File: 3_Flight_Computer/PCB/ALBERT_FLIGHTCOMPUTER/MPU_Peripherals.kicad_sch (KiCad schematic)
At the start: 27 parts, among them IC3 PCA9685PW,118, IC4 W25N01GVZEIG, J10 Screw_Terminal_01x02, J11 Screw_Terminal_01x02, J5 Conn_02x08_Odd_Even, J6 Conn_01x08, J8 Screw_Terminal_01x02, J9 Screw_Terminal_01x02, Q1 BSC028N06LS3, Q2 BSC028N06LS3, Q3 BSC028N06LS3, Q4 BSC028N06LS3

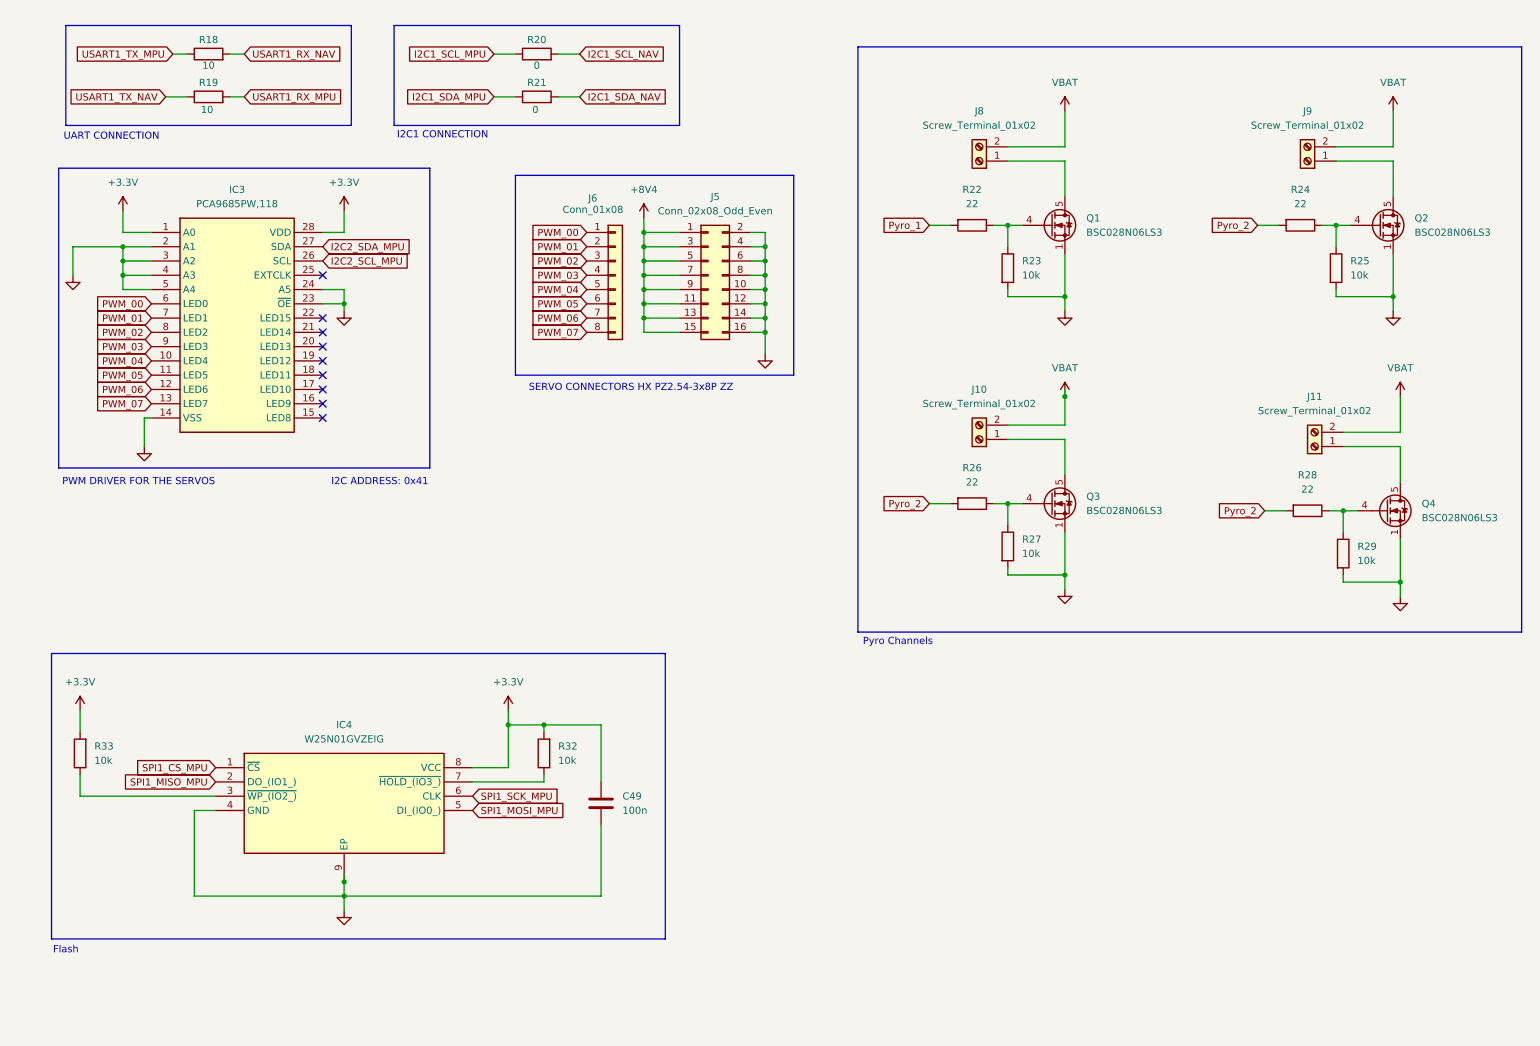
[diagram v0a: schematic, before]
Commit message: Refactor code structure for improved readability and maintainability
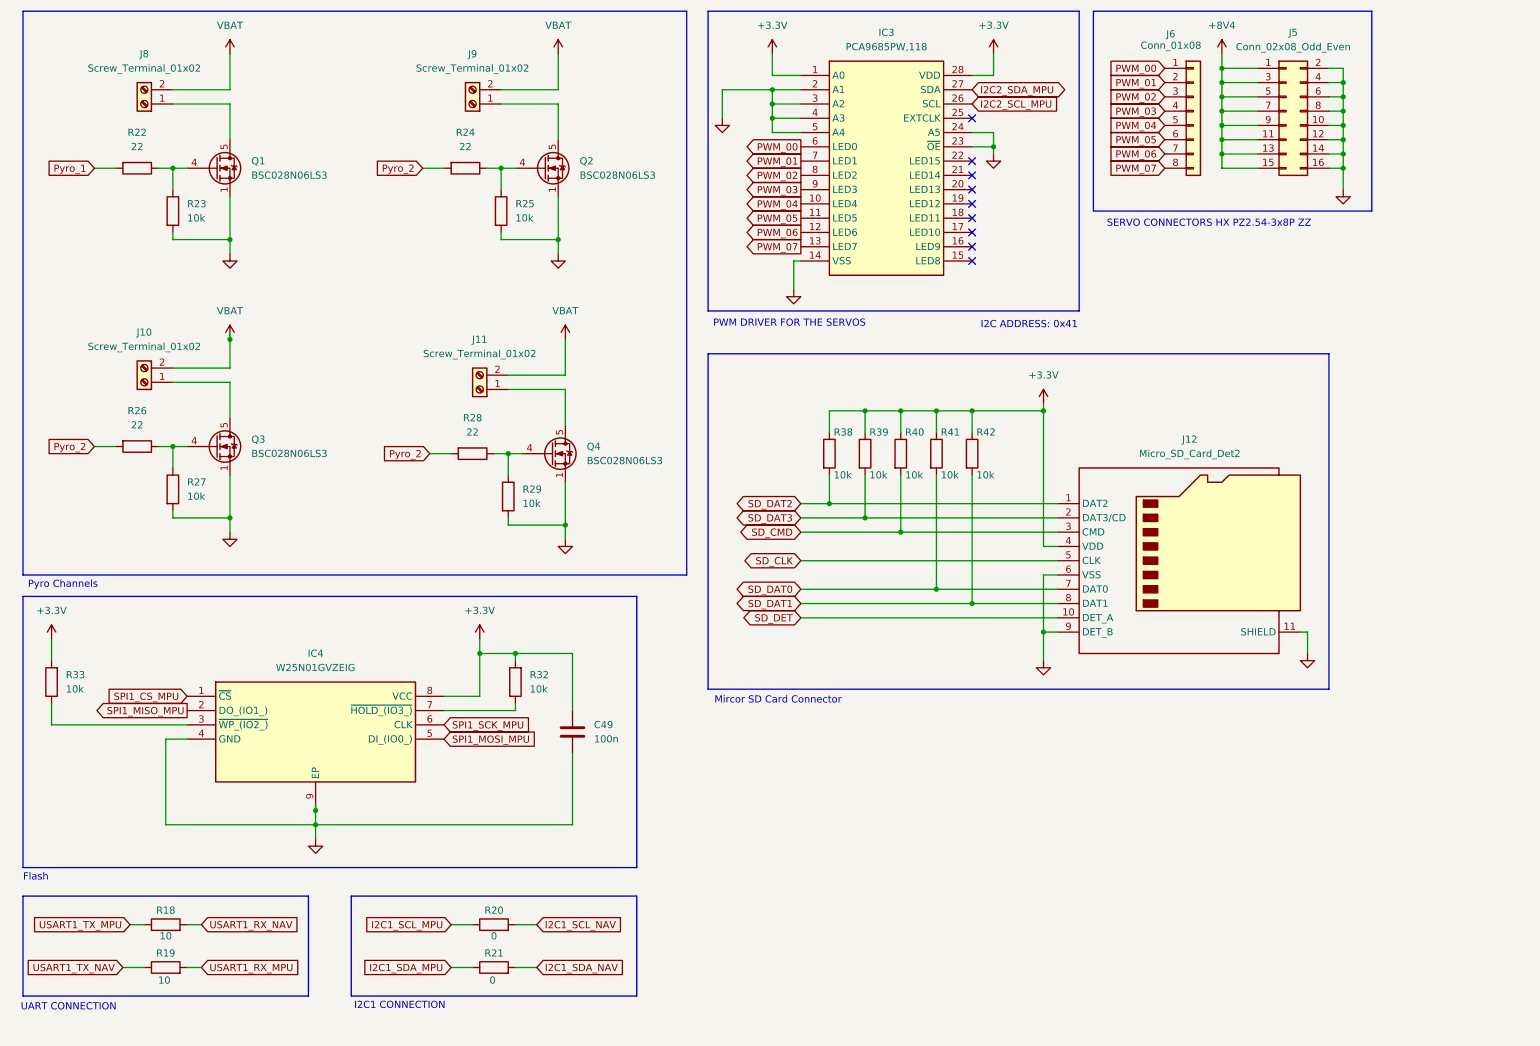
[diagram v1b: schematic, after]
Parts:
- added J12: Micro_SD_Card_Det2, Connector_Card:microSD_HC_Hirose_DM3AT-SF-PEJM5, symbol Connector:Micro_SD_Card_Det2
- added R38, R39, R40, R41, R42: 10k, symbol Device:R
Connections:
- net +3.3V: now also J12.4 (VDD), R38.1, R39.1, R40.1, R41.1, R42.1
- net GND: now also J12.11 (SHIELD), J12.6 (VSS), J12.9 (DET_B)
- new net SD_CLK: J12.5 (CLK)
- new net SD_CMD: J12.3 (CMD), R40.2
- new net SD_DAT0: J12.7 (DAT0), R41.2
- new net SD_DAT1: J12.8 (DAT1), R42.2
- new net SD_DAT2: J12.1 (DAT2), R38.2
- new net SD_DAT3: J12.2 (DAT3/CD), R39.2
- new net SD_DET: J12.10 (DET_A)
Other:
- note added: "Mircor SD Card Connector"
- title: (none) -> MPU Peripherals
- moved on the sheet: C49, IC3, IC4, J10, J11, J5, J6, J8, J9, Q1, Q2, Q3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

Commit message: Add lock file for ALBERT_FLIGHTCOMPUTER PCB design
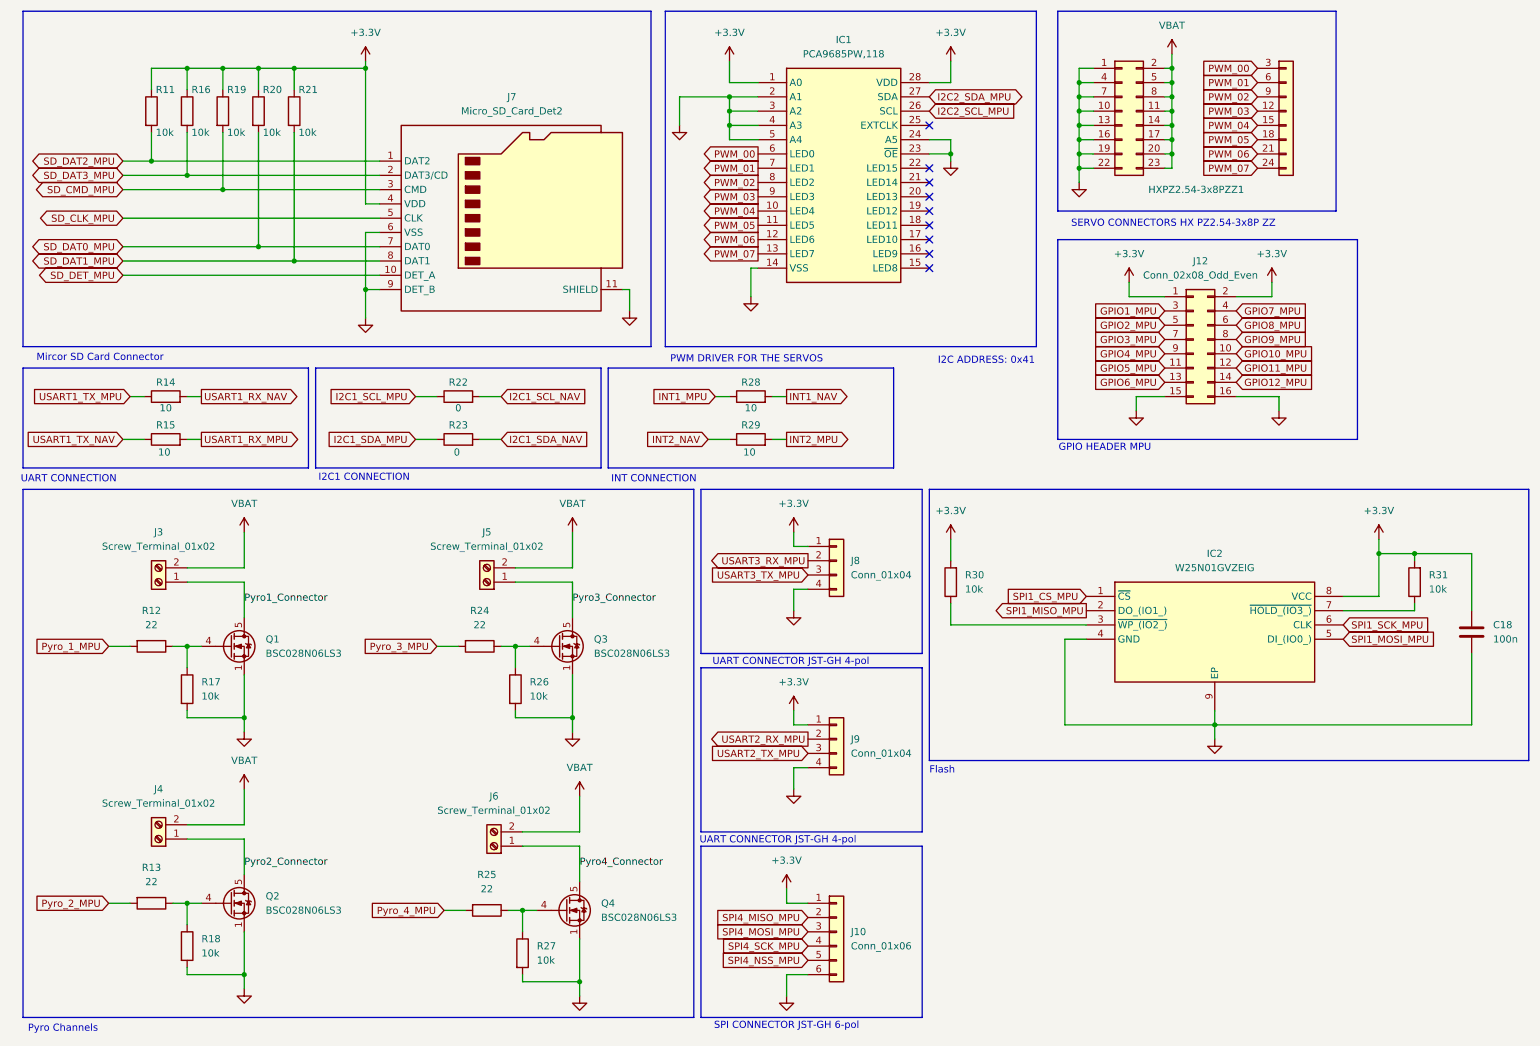
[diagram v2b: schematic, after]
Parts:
- removed J5: Conn_02x08_Odd_Even, symbol Connector_Generic:Conn_02x08_Odd_Even
- removed J6: Conn_01x08, symbol Connector_Generic:Conn_01x08
- added HXPZ2.54-3x8PZZ1: ~, HXPZ2.54-3x8PZZ:HX PZ2.54-3x8P ZZ, symbol HXPZ2.54-3x8PZZ:HXPZ2.54-3x8PZZ
- added J10: Conn_01x06, Connector_JST:JST_PH_B6B-PH-K_1x06_P2.00mm_Vertical, symbol Connector_Generic:Conn_01x06
- added J12: Conn_02x08_Odd_Even, Connector_PinHeader_2.54mm:PinHeader_2x08_P2.54mm_Vertical, symbol Connector_Generic:Conn_02x08_Odd_Even
- added J8, J9: Conn_01x04, Connector_JST:JST_PH_B4B-PH-K_1x04_P2.00mm_Vertical, symbol Connector_Generic:Conn_01x04
- added R28, R29: 10, Resistor_SMD:R_0402_1005Metric, symbol Device:R
- C18: renamed from C49; footprint (none) -> Capacitor_SMD:C_0402_1005Metric
- IC1: renamed from IC3; footprint SOP65P640X110-28N -> PCA968PW,118:SOP65P640X110-28N
- IC2: renamed from IC4; footprint SON127P800X600X80-9N-D -> W25N01GVZEIG:SON127P800X600X80-9N-D
- J3: renamed from J8; footprint (none) -> TerminalBlock_Phoenix:TerminalBlock_Phoenix_MKDS-1,5-2-5.08_1x02_P5.08mm_Horizontal
- J4: renamed from J10; footprint (none) -> TerminalBlock_Phoenix:TerminalBlock_Phoenix_MKDS-1,5-2-5.08_1x02_P5.08mm_Horizontal
- J5: renamed from J9; footprint (none) -> TerminalBlock_Phoenix:TerminalBlock_Phoenix_MKDS-1,5-2-5.08_1x02_P5.08mm_Horizontal
- J6: renamed from J11; footprint (none) -> TerminalBlock_Phoenix:TerminalBlock_Phoenix_MKDS-1,5-2-5.08_1x02_P5.08mm_Horizontal
- R11: renamed from R38; footprint (none) -> Resistor_SMD:R_0402_1005Metric
- R12: renamed from R22; footprint (none) -> Resistor_SMD:R_0402_1005Metric
- R13: renamed from R26; footprint (none) -> Resistor_SMD:R_0402_1005Metric
- R14: renamed from R18; footprint (none) -> Resistor_SMD:R_0402_1005Metric
- R15: renamed from R19; footprint (none) -> Resistor_SMD:R_0402_1005Metric
- R16: renamed from R39; footprint (none) -> Resistor_SMD:R_0402_1005Metric
- R17: renamed from R23; footprint (none) -> Resistor_SMD:R_0402_1005Metric
- R18: renamed from R27; footprint (none) -> Resistor_SMD:R_0402_1005Metric
- R19: renamed from R40; footprint (none) -> Resistor_SMD:R_0402_1005Metric
- R20: renamed from R41; footprint (none) -> Resistor_SMD:R_0402_1005Metric
- R21: renamed from R42; footprint (none) -> Resistor_SMD:R_0402_1005Metric
- R22: renamed from R20; footprint (none) -> Resistor_SMD:R_0402_1005Metric
- R23: renamed from R21; footprint (none) -> Resistor_SMD:R_0402_1005Metric
- R24: footprint (none) -> Resistor_SMD:R_0402_1005Metric
- R25: renamed from R28; footprint (none) -> Resistor_SMD:R_0402_1005Metric
- R26: renamed from R25; footprint (none) -> Resistor_SMD:R_0402_1005Metric
- R27: renamed from R29; footprint (none) -> Resistor_SMD:R_0402_1005Metric
- R30: renamed from R33; footprint (none) -> Resistor_SMD:R_0402_1005Metric
- R31: renamed from R32; footprint (none) -> Resistor_SMD:R_0402_1005Metric
- renumbered J12 to J7, Q3 to Q2, Q2 to Q3
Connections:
- net +3.3V: now also J10.1 (Pin_1), J12.1 (Pin_1), J12.2 (Pin_2), J8.1 (Pin_1), J9.1 (Pin_1)
- net GND: now also HXPZ2.54-3x8PZZ1.1, HXPZ2.54-3x8PZZ1.10, HXPZ2.54-3x8PZZ1.13, HXPZ2.54-3x8PZZ1.16, HXPZ2.54-3x8PZZ1.19, HXPZ2.54-3x8PZZ1.22, HXPZ2.54-3x8PZZ1.4, HXPZ2.54-3x8PZZ1.7, J10.6 (Pin_6), J12.15 (Pin_15), J12.16 (Pin_16), J8.4 (Pin_4), J9.4 (Pin_4)
- net PWM_00: now also HXPZ2.54-3x8PZZ1.3
- net PWM_01: now also HXPZ2.54-3x8PZZ1.6
- net PWM_02: now also HXPZ2.54-3x8PZZ1.9
- net PWM_03: now also HXPZ2.54-3x8PZZ1.12
- net PWM_04: now also HXPZ2.54-3x8PZZ1.15
- net PWM_05: now also HXPZ2.54-3x8PZZ1.18
- net PWM_06: now also HXPZ2.54-3x8PZZ1.21
- net PWM_07: now also HXPZ2.54-3x8PZZ1.24
- net VBAT: now also HXPZ2.54-3x8PZZ1.11, HXPZ2.54-3x8PZZ1.14, HXPZ2.54-3x8PZZ1.17, HXPZ2.54-3x8PZZ1.2, HXPZ2.54-3x8PZZ1.20, HXPZ2.54-3x8PZZ1.23, HXPZ2.54-3x8PZZ1.5, HXPZ2.54-3x8PZZ1.8
- net Pyro3_Connector: now reaches J5.1 (Pin_1), Q3.5 (D)
- net Pyro1_Connector: now reaches J3.1 (Pin_1), Q1.5 (D)
- net Pyro2_Connector: now reaches J4.1 (Pin_1), Q2.5 (D)
- net Pyro4_Connector: now reaches J6.1 (Pin_1), Q4.5 (D)
- net Pyro_1 renamed Pyro_1_MPU
- removed net Pyro_2: R13.2, R24.2, R25.2
- net SD_CLK renamed SD_CLK_MPU
- net SD_CMD renamed SD_CMD_MPU
- net SD_DAT0 renamed SD_DAT0_MPU
- net SD_DAT1 renamed SD_DAT1_MPU
- net SD_DAT2 renamed SD_DAT2_MPU
- net SD_DAT3 renamed SD_DAT3_MPU
- net SD_DET renamed SD_DET_MPU
- new net GPIO10_MPU: J12.10 (Pin_10)
- new net GPIO11_MPU: J12.12 (Pin_12)
- new net GPIO12_MPU: J12.14 (Pin_14)
- new net GPIO1_MPU: J12.3 (Pin_3)
- new net GPIO2_MPU: J12.5 (Pin_5)
- new net GPIO3_MPU: J12.7 (Pin_7)
- new net GPIO4_MPU: J12.9 (Pin_9)
- new net GPIO5_MPU: J12.11 (Pin_11)
- new net GPIO6_MPU: J12.13 (Pin_13)
- new net GPIO7_MPU: J12.4 (Pin_4)
- new net GPIO8_MPU: J12.6 (Pin_6)
- new net GPIO9_MPU: J12.8 (Pin_8)
- new net INT1_MPU: R28.1
- new net INT1_NAV: R28.2
- new net INT2_MPU: R29.2
- new net INT2_NAV: R29.1
- new net Pyro_2_MPU: R13.2
- new net Pyro_3_MPU: R24.2
- new net Pyro_4_MPU: R25.2
- new net SPI4_MISO_MPU: J10.2 (Pin_2)
- new net SPI4_MOSI_MPU: J10.3 (Pin_3)
- new net SPI4_NSS_MPU: J10.5 (Pin_5)
- new net SPI4_SCK_MPU: J10.4 (Pin_4)
- new net USART2_RX_MPU: J9.2 (Pin_2)
- new net USART2_TX_MPU: J9.3 (Pin_3)
- new net USART3_RX_MPU: J8.2 (Pin_2)
- new net USART3_TX_MPU: J8.3 (Pin_3)
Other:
- note added: "GPIO HEADER MPU"
- note added: "INT CONNECTION"
- note added: "SPI CONNECTOR JST-GH 6-pol"
- note added: "UART CONNECTOR JST-GH 4-pol"
- company: (none) -> ALBERT AEROSPACE
- moved on the sheet: C18, IC1, IC2, J3, J4, J5, J6, J7, Q1, Q2, Q3, Q4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
